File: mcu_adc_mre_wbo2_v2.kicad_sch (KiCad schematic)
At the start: 54 parts, among them J1 TC2030, J2 Conn_01x06_Male, J3 Conn_01x03_Male, SW1 SW_Push, U1 STM32F072CBUx, U2 MCP6004, U3 AD8628, U4 REF3033, Y1 8MHz

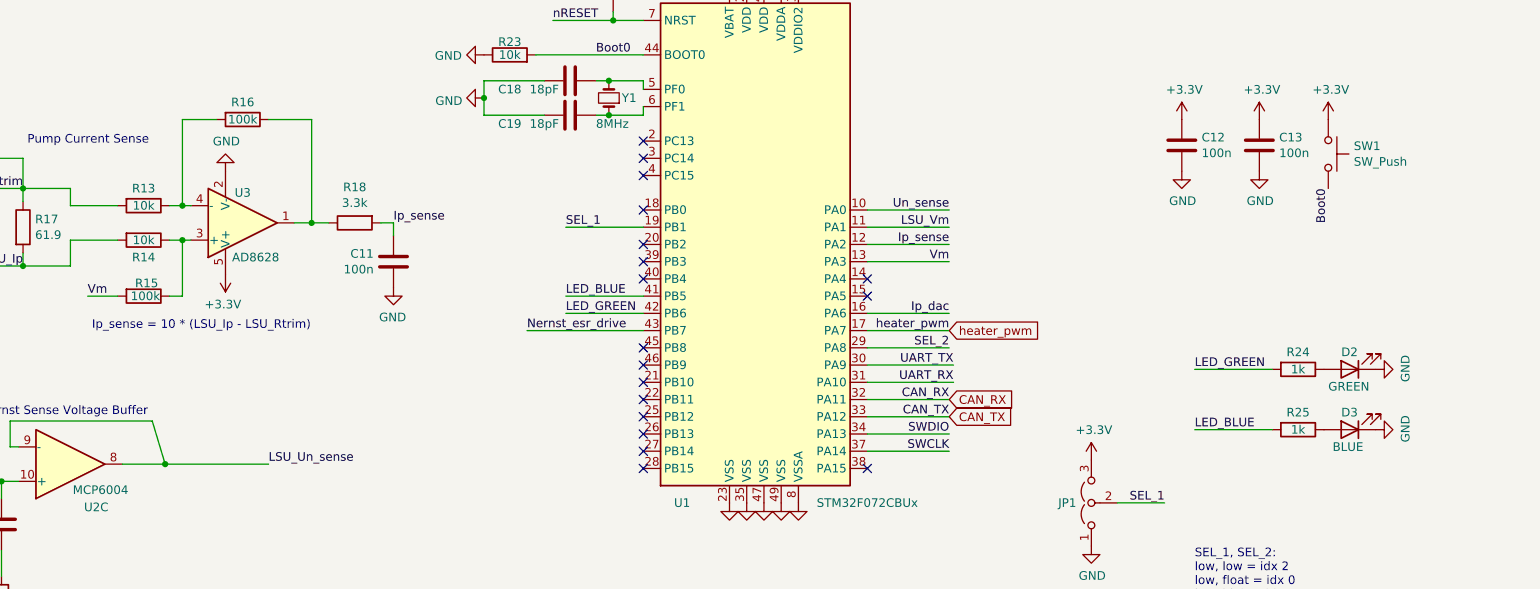
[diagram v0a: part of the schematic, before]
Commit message: V2.5 with OPAmp
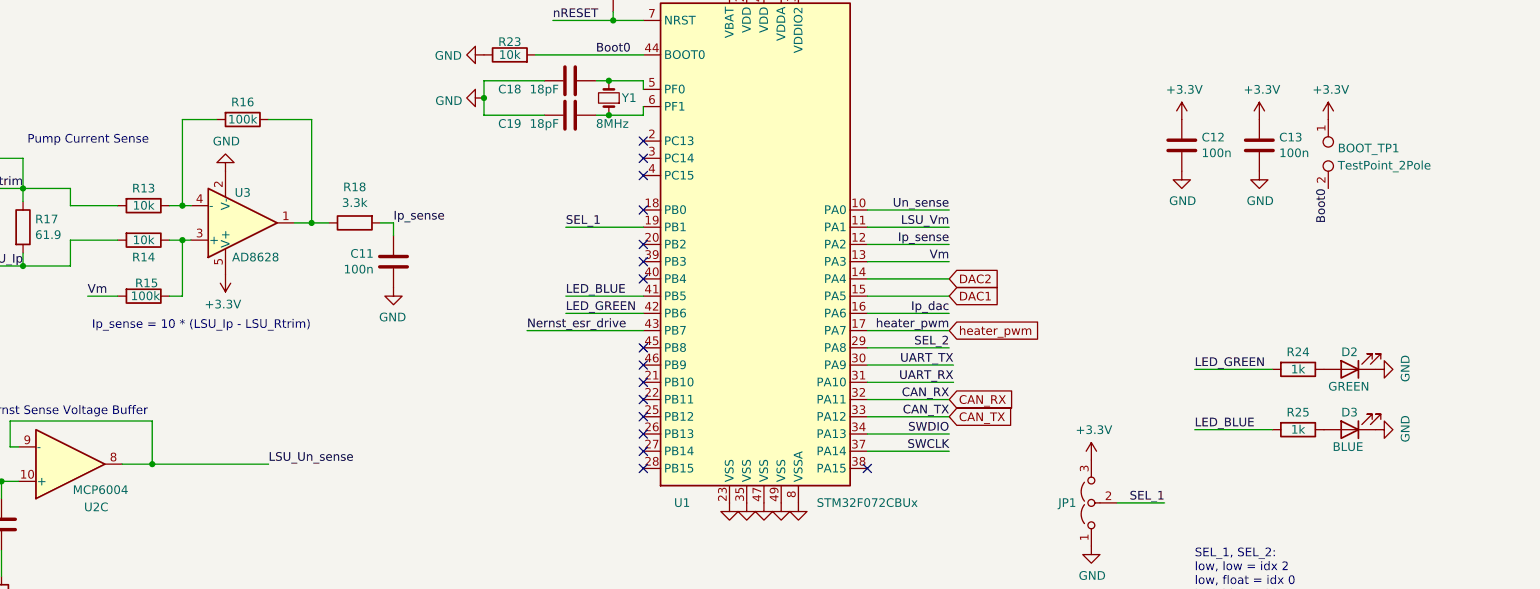
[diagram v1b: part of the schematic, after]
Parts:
- removed SW1: SW_Push, rusefi_lib:SW_SPST_CK_RS282G05A3, symbol Switch:SW_Push
- added BOOT_TP1: TestPoint_2Pole, TestPoint:TestPoint_Bridge_Pitch2.54mm_Drill0.7mm, symbol Connector:TestPoint_2Pole
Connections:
- net +3V3: now also BOOT_TP1.1
- net Boot0: now also BOOT_TP1.2
- net DAC2: now reaches U1.14 (PA4)
- net DAC1: now reaches U1.15 (PA5)
- no-connect marks 20 -> 18
